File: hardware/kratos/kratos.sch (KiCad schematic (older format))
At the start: 0 parts

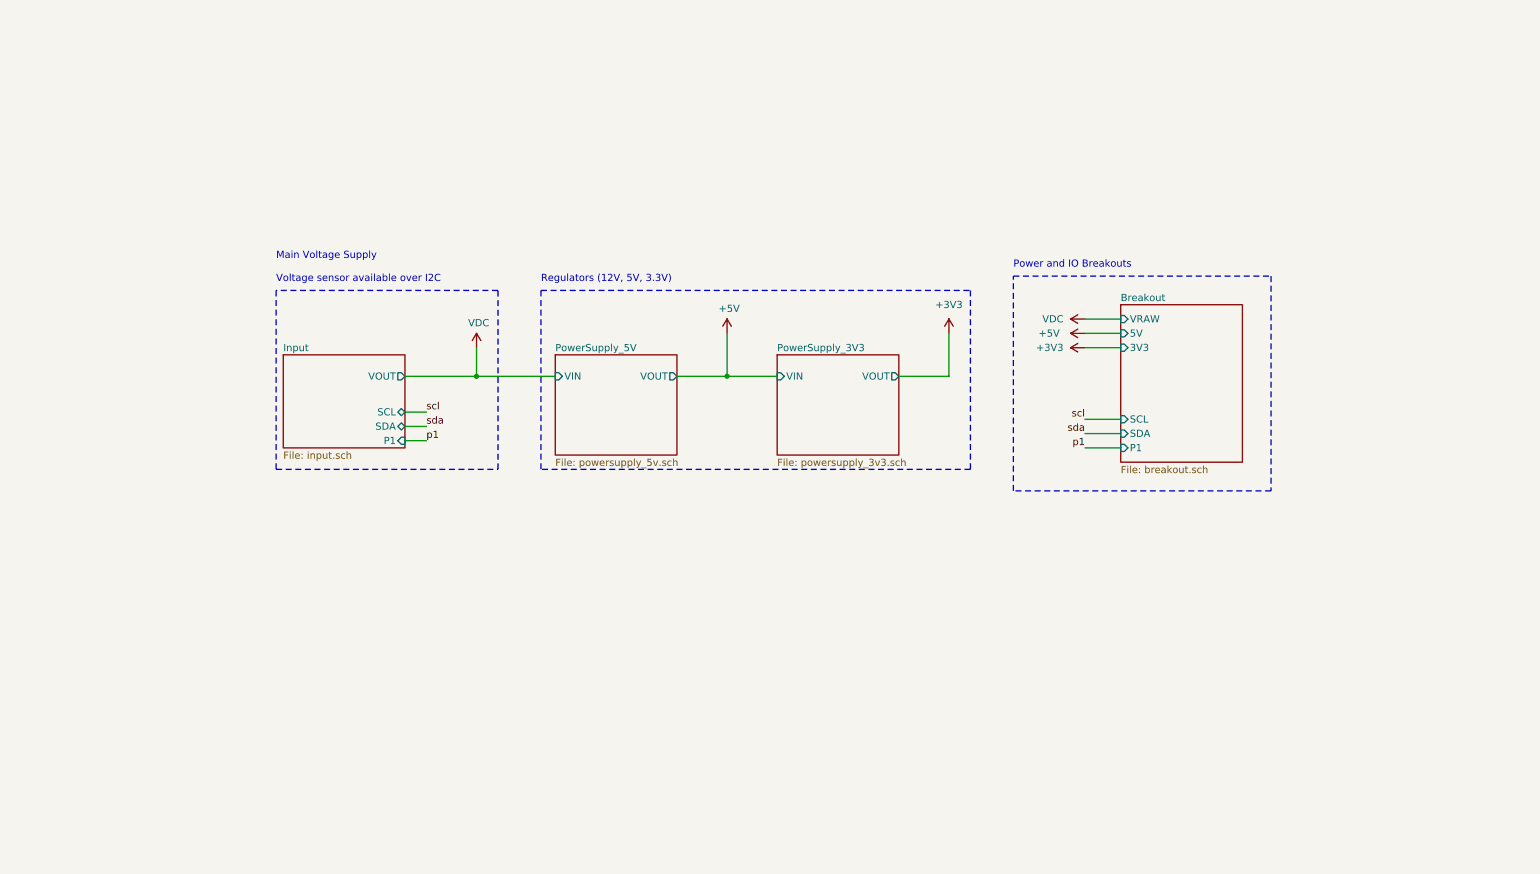
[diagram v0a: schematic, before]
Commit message: REV C
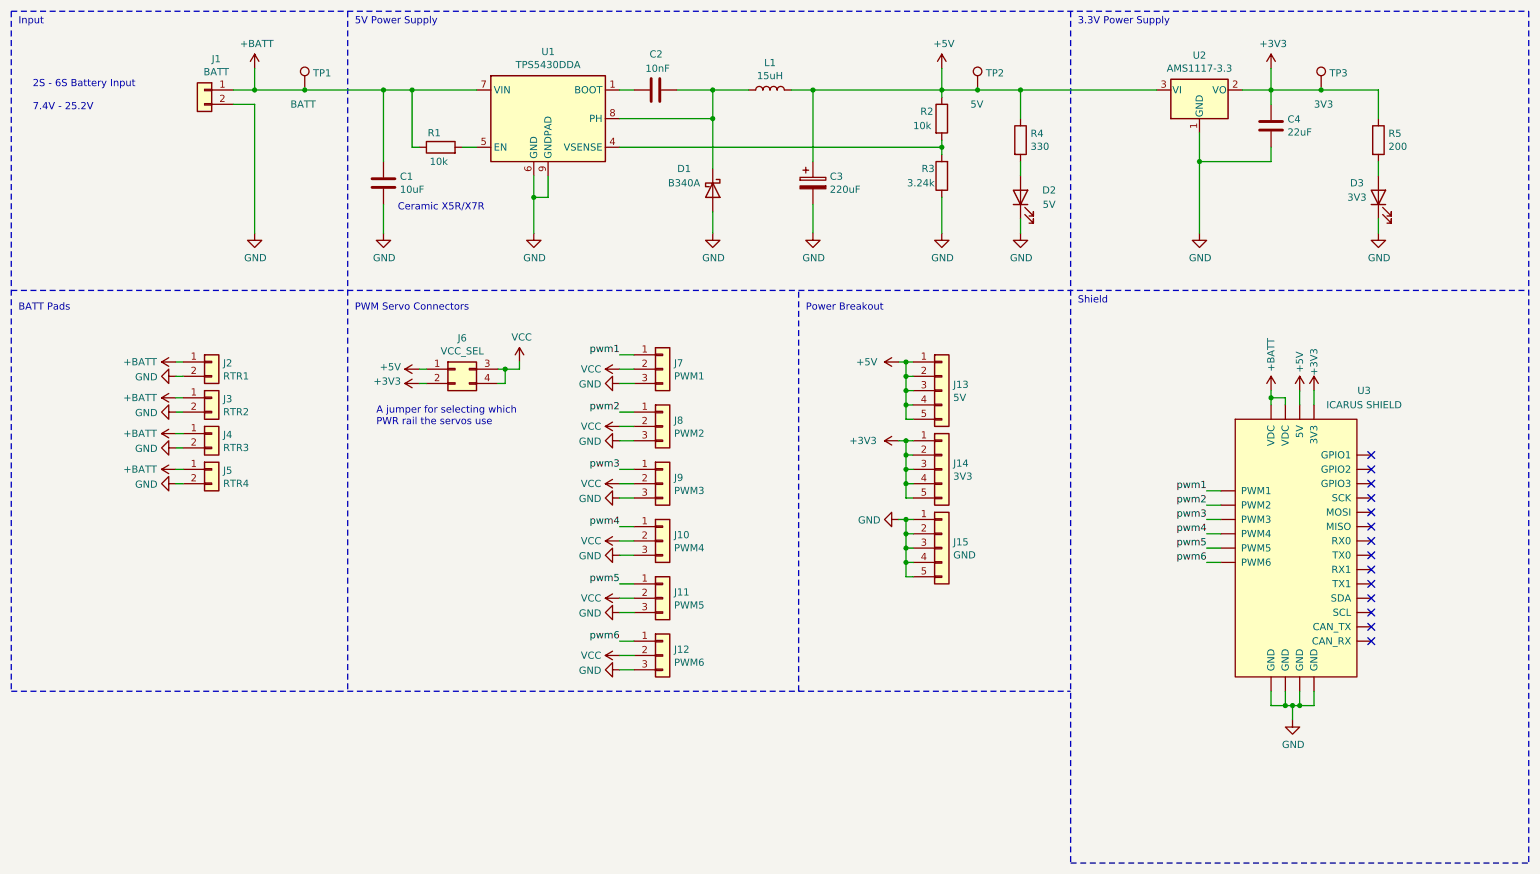
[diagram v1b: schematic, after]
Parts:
- added C1: 10uF, Capacitor_SMD:C_0805_2012Metric, symbol Device:C
- added C2: 10nF, Capacitor_SMD:C_0805_2012Metric, symbol Device:C
- added C3: 220uF, Capacitor_SMD:CP_Elec_6.3x5.4, symbol Device:CP
- added C4: 22uF, Capacitor_SMD:C_0805_2012Metric, symbol Device:C
- added D1: B340A, Diode_SMD:D_SMA, symbol Device:D_Schottky
- added D2: 5V, LED_SMD:LED_0805_2012Metric, symbol Device:LED
- added D3: 3V3, LED_SMD:LED_0805_2012Metric, symbol Device:LED
- added J1: BATT, drone:XT60, symbol Connector_Generic:Conn_01x02
- added J10: PWM4, Connector_PinSocket_2.54mm:PinSocket_1x03_P2.54mm_Vertical, symbol Connector_Generic:Conn_01x03
- added J11: PWM5, Connector_PinSocket_2.54mm:PinSocket_1x03_P2.54mm_Vertical, symbol Connector_Generic:Conn_01x03
- added J12: PWM6, Connector_PinSocket_2.54mm:PinSocket_1x03_P2.54mm_Vertical, symbol Connector_Generic:Conn_01x03
- added J13: 5V, Connector_PinSocket_2.54mm:PinSocket_1x05_P2.54mm_Vertical, symbol Connector_Generic:Conn_01x05
- added J14: 3V3, Connector_PinSocket_2.54mm:PinSocket_1x05_P2.54mm_Vertical, symbol Connector_Generic:Conn_01x05
- added J15: GND, Connector_PinSocket_2.54mm:PinSocket_1x05_P2.54mm_Vertical, symbol Connector_Generic:Conn_01x05
- added J2: RTR1, drone:XT60, symbol Connector_Generic:Conn_01x02
- added J3: RTR2, drone:XT60, symbol Connector_Generic:Conn_01x02
- added J4: RTR3, drone:XT60, symbol Connector_Generic:Conn_01x02
- added J5: RTR4, drone:XT60, symbol Connector_Generic:Conn_01x02
- added J6: VCC_SEL, Connector_PinSocket_2.54mm:PinSocket_2x02_P2.54mm_Vertical, symbol Connector_Generic:Conn_02x02_Top_Bottom
- added J7: PWM1, Connector_PinSocket_2.54mm:PinSocket_1x03_P2.54mm_Vertical, symbol Connector_Generic:Conn_01x03
- added J8: PWM2, Connector_PinSocket_2.54mm:PinSocket_1x03_P2.54mm_Vertical, symbol Connector_Generic:Conn_01x03
- added J9: PWM3, Connector_PinSocket_2.54mm:PinSocket_1x03_P2.54mm_Vertical, symbol Connector_Generic:Conn_01x03
- added L1: 15uH, inductors:MWSA0603S-150MT, symbol Device:L
- added R1, R2: 10k, Resistor_SMD:R_0805_2012Metric, symbol Device:R
- added R3: 3.24k, Resistor_SMD:R_0805_2012Metric, symbol Device:R
- added R4: 330, Resistor_SMD:R_0805_2012Metric, symbol Device:R
- added R5: 200, Resistor_SMD:R_0805_2012Metric, symbol Device:R
- added TP1: BATT, TestPoint:TestPoint_Pad_2.0x2.0mm, symbol Connector:TestPoint
- added TP2: 5V, TestPoint:TestPoint_Pad_2.0x2.0mm, symbol Connector:TestPoint
- added TP3: 3V3, TestPoint:TestPoint_Pad_2.0x2.0mm, symbol Connector:TestPoint
- added U1: TPS5430DDA, Package_SO:TI_SO-PowerPAD-8_ThermalVias, symbol Regulator_Switching:TPS5430DDA
- added U2: AMS1117-3.3, Package_TO_SOT_SMD:SOT-223-3_TabPin2, symbol Regulator_Linear:AMS1117-3.3
- added U3: ICARUS SHIELD, icarus:icarus-shield, symbol icarus:ICARUS
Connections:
- net +3V3: now also C4.1, J14.1 (Pin_1), J14.2 (Pin_2), J14.3 (Pin_3), J14.4 (Pin_4), J14.5 (Pin_5), J6.2 (Pin_2), R5.1, TP3.1, U2.2 (VO), U3.7 (3V3)
- net +5V: now also C3.1, J13.1 (Pin_1), J13.2 (Pin_2), J13.3 (Pin_3), J13.4 (Pin_4), J13.5 (Pin_5), J6.1 (Pin_1), L1.2, R2.1, R4.1, TP2.1, U2.3 (VI), U3.5 (5V)
- new net: C2.1, U1.1 (BOOT)
- new net: C2.2, D1.1 (K), L1.1, U1.8 (PH)
- new net: R2.2, R3.2, U1.4 (VSENSE)
- new net: R1.2, U1.5 (EN)
- new net: D2.2 (A), R4.2
- new net: D3.2 (A), R5.2
- new net +BATT: C1.1, J1.1 (Pin_1), J2.1 (Pin_1), J3.1 (Pin_1), J4.1 (Pin_1), J5.1 (Pin_1), R1.1, TP1.1, U1.7 (VIN), U3.1 (VDC), U3.3 (VDC)
- new net GND: C1.2, C3.2, C4.2, D1.2 (A), D2.1 (K), D3.1 (K), J1.2 (Pin_2), J10.3 (Pin_3), J11.3 (Pin_3), J12.3 (Pin_3), J15.1 (Pin_1), J15.2 (Pin_2), J15.3 (Pin_3), J15.4 (Pin_4), J15.5 (Pin_5), J2.2 (Pin_2), J3.2 (Pin_2), J4.2 (Pin_2), J5.2 (Pin_2), J7.3 (Pin_3), J8.3 (Pin_3), J9.3 (Pin_3), R3.1, U1.6 (GND), U1.9 (GNDPAD), U2.1 (GND), U3.2 (GND), U3.4 (GND), U3.6 (GND), U3.8 (GND)
- new net VCC: J10.2 (Pin_2), J11.2 (Pin_2), J12.2 (Pin_2), J6.3 (Pin_3), J6.4 (Pin_4), J7.2 (Pin_2), J8.2 (Pin_2), J9.2 (Pin_2)
- new net pwm1: J7.1 (Pin_1), U3.9 (PWM1)
- new net pwm2: J8.1 (Pin_1), U3.10 (PWM2)
- new net pwm3: J9.1 (Pin_1), U3.11 (PWM3)
- new net pwm4: J10.1 (Pin_1), U3.12 (PWM4)
- new net pwm5: J11.1 (Pin_1), U3.13 (PWM5)
- new net pwm6: J12.1 (Pin_1), U3.14 (PWM6)
- no-connect marks 0 -> 14
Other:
- note added: "2S - 6S Battery Input\n\n7.4V - 25.2V\n"
- note added: "3.3V Power Supply"
- note added: "5V Power Supply"
- note added: "A jumper for selecting which\nPWR rail the servos use"
- note added: "BATT Pads"
- note added: "Ceramic X5R/X7R"
- note added: "Input"
- note added: "PWM Servo Connectors"
- note added: "Power Breakout"
- note added: "Shield"
- note removed: "Main Voltage Supply\n\nVoltage sensor available over I2C\n"
- note removed: "Power and IO Breakouts"
- note removed: "Regulators (12V, 5V, 3.3V)"
